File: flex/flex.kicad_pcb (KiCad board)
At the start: 2 copper layers, 126.3 x 90.6 mm, 85 parts, among them J1 Conn_01x04_Female, J2 Conn_01x05_Female, J3 Conn_01x03_Female, J4 Conn_01x06_Female, J5 Conn_01x03_Female, SW10 SW_Push, SW11 SW_Push, SW12 SW_Push, SW15 SW_Push, SW16 SW_Push, SW17 SW_Push, SW2 SW_Push, SW20 SW_Push, SW21 SW_Push, SW22 SW_Push, SW24 SW_Push, SW25 SW_Push, SW26 SW_Push, SW3 SW_Push, SW4 SW_Push, SW6 SW_Push, SW7 SW_Push, SW8 SW_Push

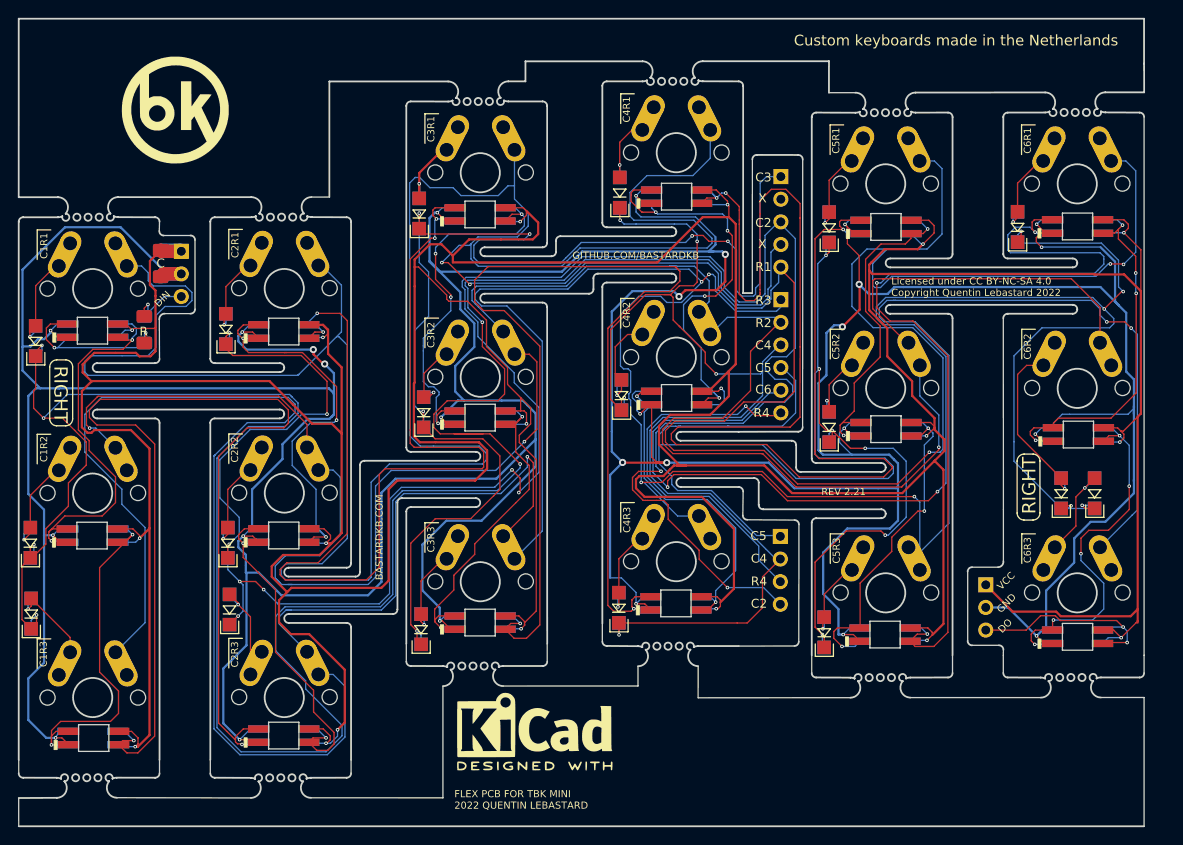
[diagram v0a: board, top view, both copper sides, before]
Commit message: bork
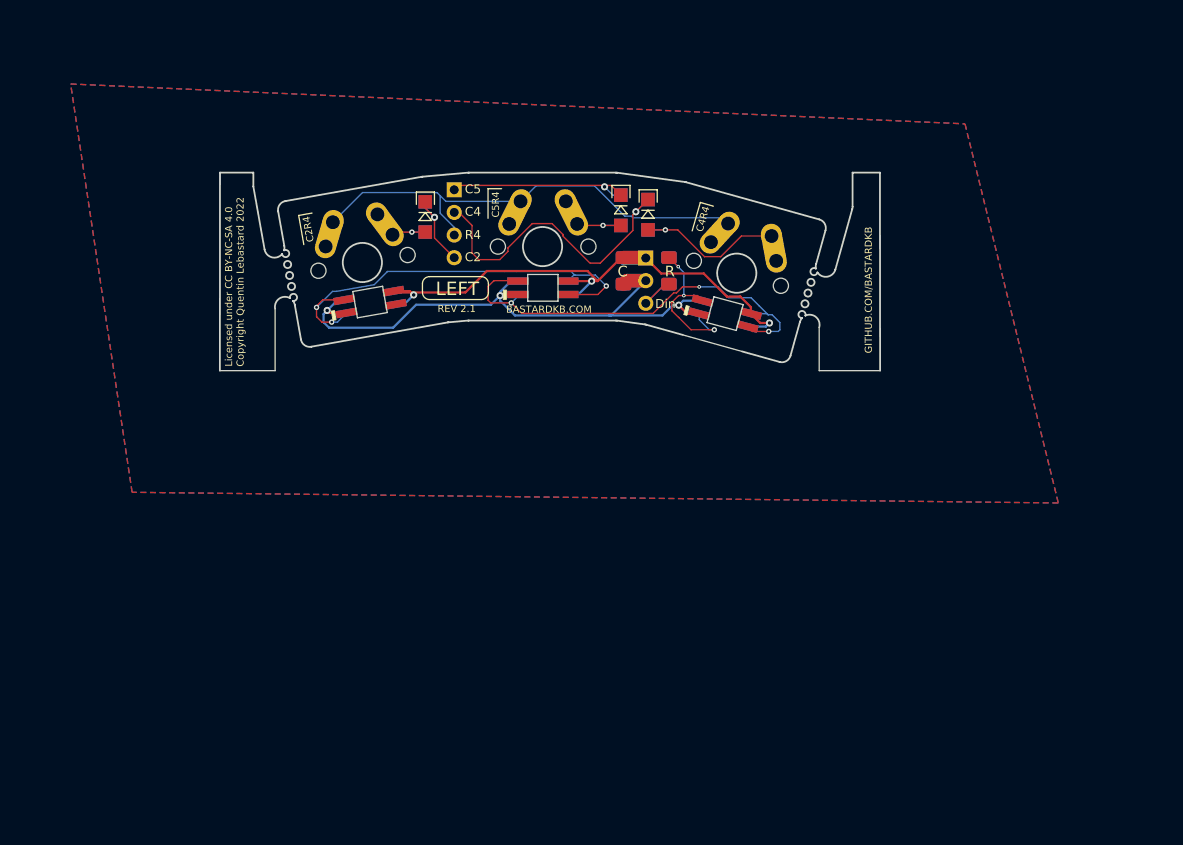
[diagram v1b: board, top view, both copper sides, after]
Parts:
- removed D1, D15, D16, D17, D2, D20, D27, D31, D32, D35, D36, D9: D, custom:Diode_TH_SOD123
- removed D18, D21, D23, D25, D3, D33, D37, D39, D4, D41, D47, D49, D51, D55, D57, D59: SK6812MINI, libs2:YS-SK6812MINI-E_REVERSE
- removed D22, D24, D26, D28, D29, D30, D34, D38, D40, D42, D48, D50, D52, D56, D58, D6, D60: SK6812MINI, libs2:YS-SK6812MINI-E_REVERSE_NO_EDGECUT
- removed G*** (x4): LOGO, LOGO
- removed J3, J5: Conn_01x03_Female, Connector_PinHeader_2.54mm:PinHeader_1x03_P2.54mm_Vertical
- removed J4: Conn_01x06_Female, Connector_PinHeader_2.54mm:PinHeader_1x06_P2.54mm_Vertical
- removed SW10, SW11, SW12, SW15, SW16, SW17, SW2, SW20, SW21, SW22, SW24, SW25, SW26, SW3, SW4, SW6, SW7, SW8: SW_Push, custom:SW_MX_reversible
- added SW14: SW_Push, custom:SW_MX_reversible, F.Cu at (116.1, 77.6)
- added SW19: SW_Push, custom:SW_MX_reversible, F.Cu at (94.3, 74.6)
- added SW5: SW_Push, custom:SW_MX_reversible, F.Cu at (74.1, 76.4)
- C1, C2: footprint Capacitor_SMD:C_1206_3216Metric_Pad1.42x1.75mm_HandSolder -> LED_SMD:LED_1206_3216Metric_Pad1.42x1.75mm_HandSolder
- D10, D12: value D -> SK6812MINI; footprint custom:Diode_TH_SOD123 -> libs2:YS-SK6812MINI-E_REVERSE
- D11, D13: value D -> SK6812MINI; footprint custom:Diode_TH_SOD123 -> libs2:YS-SK6812MINI-E_REVERSE_NO_EDGECUT; moved to B.Cu
- D5: value SK6812MINI -> D; footprint libs2:YS-SK6812MINI-E_REVERSE -> custom:Diode_TH_SOD123
- J2: value Conn_01x05_Female -> Conn_01x03_Female; footprint customs:PinHeader_1x05_P2.54mm_Vertical -> Connector_PinHeader_2.54mm:PinHeader_1x03_P2.54mm_Vertical
- moved D10 66.6 mm to (94.2, 79.2), turned to 0 degrees
- moved D5 65.2 mm to (81.0, 66.2), turned to -90 degrees
- moved R2 59.3 mm to (108.4, 77.3)
- moved R1 59.2 mm to (108.4, 77.3)
- moved D7 55.4 mm to (114.7, 82.1), turned to -15 degrees
- moved D8 55.4 mm to (114.7, 82.1), turned to -15 degrees
- moved J1 53.4 mm to (84.3, 68.2)
- moved C1 52.0 mm to (103.3, 77.3)
- moved C2 51.9 mm to (103.3, 77.3)
- moved D12 42.5 mm to (74.8, 80.8), turned to 10 degrees
- moved D19 39.5 mm to (103.0, 65.5), turned to -90 degrees
- moved D13 29.0 mm to (74.8, 80.8), turned to 10 degrees
- moved D14 23.3 mm to (106.0, 66.0), turned to -90 degrees
- moved J2 17.7 mm to (105.8, 75.9)
- moved D11 14.3 mm to (94.2, 79.2), turned to 0 degrees
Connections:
- D10 pad 1: col1 -> Net-(D10-Pad1)
- D10 pad 2: Net-(D10-Pad2) -> Gnd
- D11 pad 1: col3 -> Net-(D10-Pad1)
- D11 pad 2: Net-(D11-Pad2) -> Gnd
- D12 pad 1: col2 -> Net-(D12-Pad1)
- D12 pad 2: Net-(D12-Pad2) -> Gnd
- D13 pad 1: col4 -> Net-(D13-Pad1)
- D13 pad 2: Net-(D13-Pad2) -> Gnd
- D14 pad 1: col5 -> col4
- D19 pad 1: col3 -> col5
- D5 pad 1: Net-(D5-Pad1) -> col2
- D5 pad 2: Gnd -> Net-(D5-Pad2)
- D7 pad 1: Net-(D33-Pad3) -> Net-(D10-Pad3)
- D7 pad 3: Net-(D5-Pad1) -> Net-(D7-Pad3)
- D8 pad 1: Net-(D33-Pad3) -> Net-(D10-Pad3)
- D8 pad 3: Net-(D5-Pad1) -> Net-(D7-Pad3)
- J1 pad 3: row5 -> row1
- J2 pad 1: col3 -> Vcc
- J2 pad 2: Net-(J2-Pad2) -> Gnd
- J2 pad 3: col2 -> Din
- R1 pad 1: Din -> Net-(D7-Pad3)
- R1 pad 2: Net-(D28-Pad3) -> Din
- R2 pad 1: Din -> Net-(D7-Pad3)
- R2 pad 2: Net-(D28-Pad3) -> Din
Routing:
- net Vcc: track 702.6 -> 67.5 mm, vias 19 -> 3
- net Gnd: track 699.9 -> 71.1 mm, vias 27 -> 3
- net row2: track 481.4 -> 0.00 mm, vias 5 -> 0
- net row4: track 431.6 -> 0.00 mm, vias 7 -> 0
- net col1: track 278.4 -> 0.00 mm, vias 6 -> 0
- net row3: track 265.4 -> 0.00 mm, vias 3 -> 0
- net col2: track 256.2 -> 9.78 mm, vias 10 -> 1
- net col6: track 174.7 -> 0.00 mm, vias 7 -> 0
- net Net-(D41-Pad1): track 147.8 -> 0.00 mm, vias 3 -> 0
- net col3: track 143.7 -> 0.00 mm, vias 6 -> 0
- net col5: track 158.5 -> 21.5 mm, vias 6 -> 1
- net Net-(D25-Pad1): track 127.8 -> 0.00 mm, vias 2 -> 0
- net Net-(D18-Pad1): track 124.7 -> 0.00 mm, vias 2 -> 0
- net Net-(D21-Pad3): track 120.4 -> 0.00 mm, vias 4 -> 0
- net Net-(D51-Pad1): track 103.0 -> 0.00 mm, vias 3 -> 0
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- added copper zone on B.Cu, net Gnd
- added copper zone on F.Cu, net Gnd
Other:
- board size 126.3 x 90.6 mm -> 74.1 x 22.2 mm
- board text added: "C2R4"
- board text added: "C4R4"
- board text added: "C5R4"
- board text added: "Din"
- board text added: "REV 2.1"
- board text removed: "C1R1"
- board text removed: "C1R2"
- board text removed: "C1R3"
- board text removed: "C2R1"
- board text removed: "C2R2"
- board text removed: "C2R3"
- board text removed: "C3"
- board text removed: "C3R1"
- board text removed: "C3R2"
- board text removed: "C3R3"
- board text removed: "C4R1"
- board text removed: "C4R2"
- board text removed: "C4R3"
- board text removed: "C5R1"
- board text removed: "C5R2"
- board text removed: "C5R3"
- board text removed: "C6"
- board text removed: "C6R1"
- board text removed: "C6R2"
- board text removed: "C6R3"
- board text removed: "Custom keyboards made in the Netherlands"
- board text removed: "DIN"
- board text removed: "DO"
- board text removed: "FLEX PCB FOR TBK MINI 2022 QUENTIN LEBASTARD"
- board text removed: "GND"
- board text removed: "R1"
- board text removed: "R2"
- board text removed: "R3"
- board text removed: "REV 2.21"
- board text removed: "VCC"
- board text removed: "X"
